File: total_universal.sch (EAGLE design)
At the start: 31 parts, among them IC1 MCP602P, M1 ARDUINO-NANO-3.0, Q1 IRFZ44n, Q2 2N2907, T1 2N2222

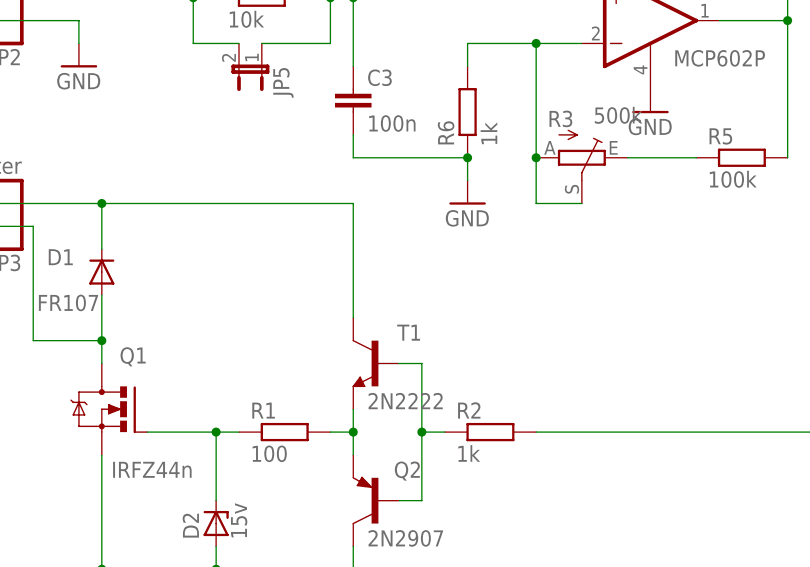
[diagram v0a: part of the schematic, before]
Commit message: Add files via upload
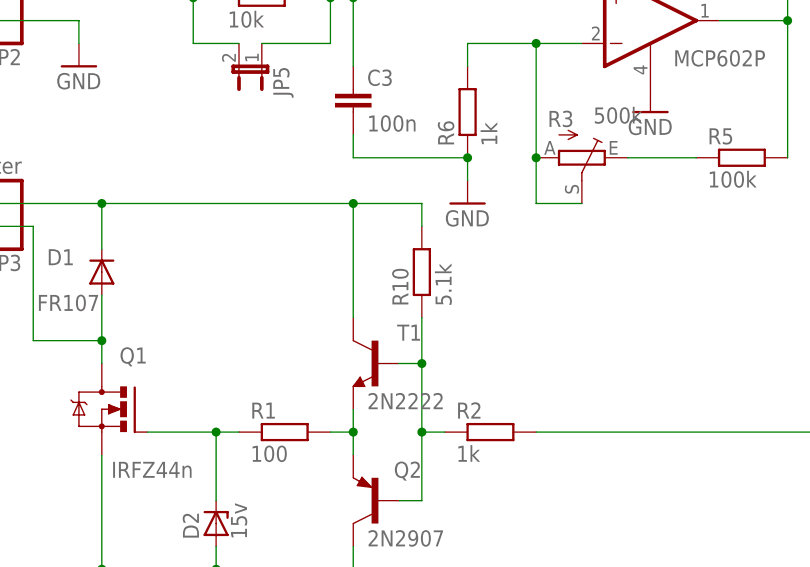
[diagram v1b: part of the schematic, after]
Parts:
- added R10: 5.1k, rcl:R-EU_0204/5
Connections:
- net N$1: now also R10.2
- net N$8: now also R10.1
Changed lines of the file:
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@@
 <part name="JP6" library="jumper" library_urn="urn:adsk.eagle:library:252" deviceset="JP1E" device="" package3d_urn="urn:adsk.eagle:package:15455/1"/>
 <part name="R9" library="rcl" library_urn="urn:adsk.eagle:library:334" deviceset="R-EU_" device="0204/5" package3d_urn="urn:adsk.eagle:package:23488/1" value="100k"/>
+<part name="R10" library="rcl" library_urn="urn:adsk.eagle:library:334" deviceset="R-EU_" device="0204/5" package3d_urn="urn:adsk.eagle:package:23488/1" value="5.1k"/>
 </parts>
 <sheets>
@@
 <attribute name="VALUE" x="24.13" y="55.118" size="1.778" layer="96"/>
 </instance>
+<instance part="R10" gate="G$1" x="25.4" y="20.32" rot="R90">
+<attribute name="NAME" x="23.9014" y="16.51" size="1.778" layer="95" rot="R90"/>
+<attribute name="VALUE" x="28.702" y="16.51" size="1.778" layer="96" rot="R90"/>
+</instance>
 </instances>
 <busses>
@@
 <wire x1="17.78" y1="27.94" x2="-10.16" y2="27.94" width="0.1524" layer="91"/>
 <junction x="-10.16" y="27.94"/>
+<pinref part="R10" gate="G$1" pin="2"/>
+<wire x1="25.4" y1="25.4" x2="25.4" y2="27.94" width="0.1524" layer="91"/>
+<wire x1="25.4" y1="27.94" x2="17.78" y2="27.94" width="0.1524" layer="91"/>
+<junction x="17.78" y="27.94"/>
 </segment>
 </net>
@@
 <wire x1="27.94" y1="2.54" x2="25.4" y2="2.54" width="0.1524" layer="91"/>
 <junction x="25.4" y="2.54"/>
-</segment>
-</net>
+<pinref part="R10" gate="G$1" pin="1"/>
+<wire x1="25.4" y1="10.16" x2="25.4" y2="15.24" width="0.1524" layer="91"/>
+<junction x="25.4" y="10.16"/>
+</segment>
+</net>

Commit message: Add files via upload
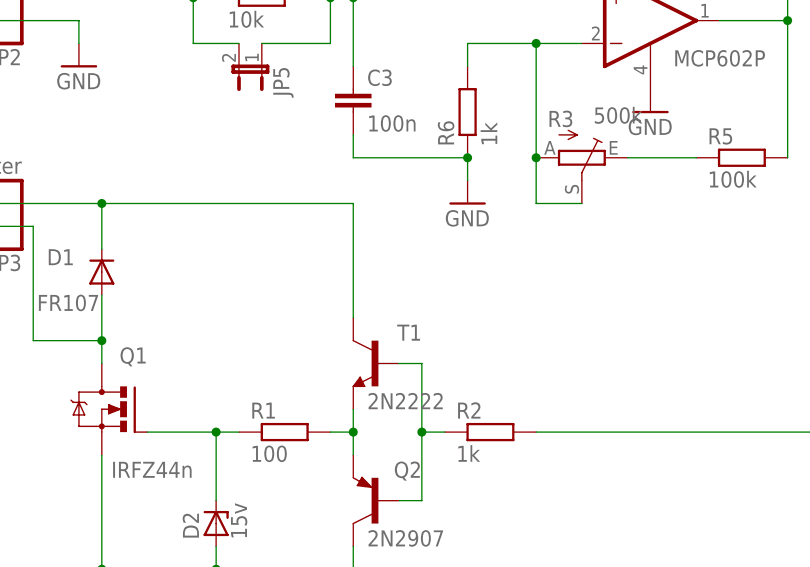
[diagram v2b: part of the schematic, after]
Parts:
- removed R10: 5.1k, rcl:R-EU_0204/5
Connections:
- net N$1: no longer R10.2
- net N$8: no longer R10.1
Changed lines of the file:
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@@
 <part name="JP6" library="jumper" library_urn="urn:adsk.eagle:library:252" deviceset="JP1E" device="" package3d_urn="urn:adsk.eagle:package:15455/1"/>
 <part name="R9" library="rcl" library_urn="urn:adsk.eagle:library:334" deviceset="R-EU_" device="0204/5" package3d_urn="urn:adsk.eagle:package:23488/1" value="100k"/>
-<part name="R10" library="rcl" library_urn="urn:adsk.eagle:library:334" deviceset="R-EU_" device="0204/5" package3d_urn="urn:adsk.eagle:package:23488/1" value="5.1k"/>
 </parts>
 <sheets>
@@
 <attribute name="VALUE" x="24.13" y="55.118" size="1.778" layer="96"/>
 </instance>
-<instance part="R10" gate="G$1" x="25.4" y="20.32" rot="R90">
-<attribute name="NAME" x="23.9014" y="16.51" size="1.778" layer="95" rot="R90"/>
-<attribute name="VALUE" x="28.702" y="16.51" size="1.778" layer="96" rot="R90"/>
-</instance>
 </instances>
 <busses>
@@
 <wire x1="17.78" y1="27.94" x2="-10.16" y2="27.94" width="0.1524" layer="91"/>
 <junction x="-10.16" y="27.94"/>
-<pinref part="R10" gate="G$1" pin="2"/>
-<wire x1="25.4" y1="25.4" x2="25.4" y2="27.94" width="0.1524" layer="91"/>
-<wire x1="25.4" y1="27.94" x2="17.78" y2="27.94" width="0.1524" layer="91"/>
-<junction x="17.78" y="27.94"/>
 </segment>
 </net>
@@
 <wire x1="27.94" y1="2.54" x2="25.4" y2="2.54" width="0.1524" layer="91"/>
 <junction x="25.4" y="2.54"/>
-<pinref part="R10" gate="G$1" pin="1"/>
-<wire x1="25.4" y1="10.16" x2="25.4" y2="15.24" width="0.1524" layer="91"/>
-<junction x="25.4" y="10.16"/>
-</segment>
-</net>
+</segment>
+</net>
